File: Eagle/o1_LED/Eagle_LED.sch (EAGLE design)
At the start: 10 parts, among them Q1 S9013

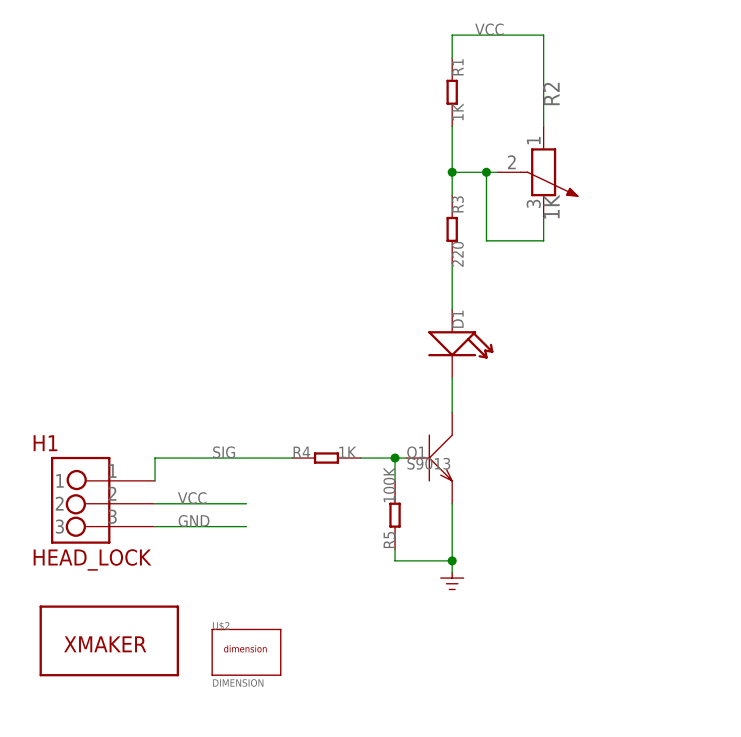
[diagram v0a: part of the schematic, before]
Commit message: miniuno
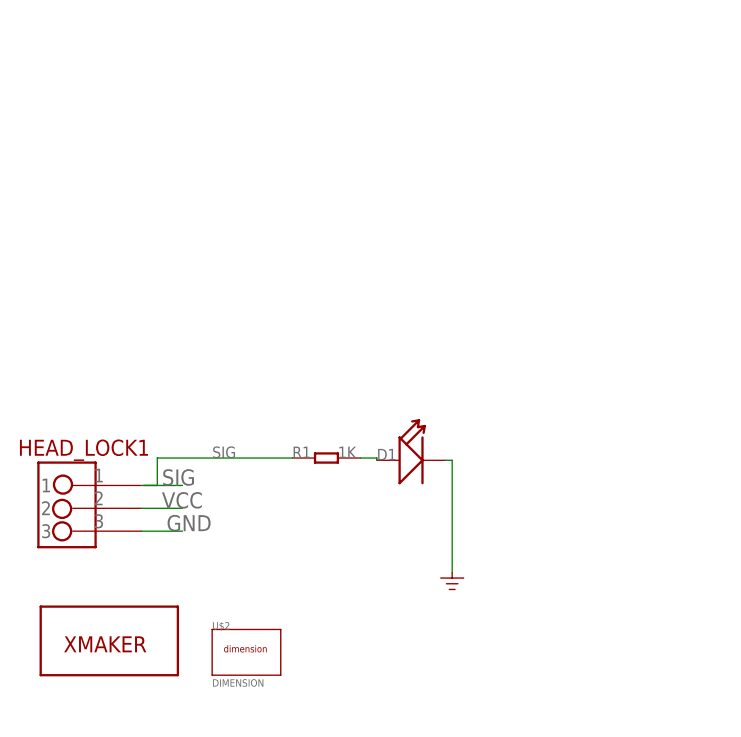
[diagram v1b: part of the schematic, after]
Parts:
- removed H1: HEAD_LOCK, HEAD_LOCK:HEAD_LOCK
- removed Q1: S9013, Discrete:TRANSISTOR-NPN-SOT23
- removed R2: 1K, Discrete:R-POTENTIOMETER'EVN-D8A-A03-B**'
- removed R3: 220, Discrete:005-R0603
- removed R4: 1K, Discrete:005-R0603
- removed R5: 100K, Discrete:005-R0603
- added HEAD_LOCK1: HEAD_LOCK, Xmaker_yuhuilbr:HEAD_LOCK
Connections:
- removed net N$2: D1.-, Q1.C
- removed net N$3: D1.+, R3.2
- removed net N$4: Q1.B, R4.2, R5.2
- net GND: now also D1.-, HEAD_LOCK1.3; no longer H1.3, Q1.E, R5.1
- net N$1: now also D1.+; no longer R2.2, R2.3, R3.1
- net SIG: now also HEAD_LOCK1.1, R1.1; no longer H1.1, R4.1
- net VCC: now also HEAD_LOCK1.2; no longer H1.2, R1.1, R2.1
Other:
- moved on the sheet: D1, R1
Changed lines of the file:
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@@
 <setting verticaltext="up"/>
 </settings>
-<grid distance="0.1" unitdist="inch" unit="inch" style="lines" multiple="1" display="no" altdistance="0.01" altunitdist="inch" altunit="inch"/>
+<grid distance="10" unitdist="mil" unit="mil" style="lines" multiple="1" display="no" altdistance="0.01" altunitdist="inch" altunit="inch"/>
 <layers>
 <layer number="1" name="Top" color="4" fill="1" visible="no" active="no"/>
@@
 <parts>
 <part name="U$1" library="moudle" deviceset="SEEEDSTUDIO_SCH_FRAME" device=""/>
+<part name="D1" library="Discrete" deviceset="LED*" device="-6MM"/>
+<part name="U$3" library="Power or GND " deviceset="GND_POWER" device=""/>
 <part name="R1" library="Discrete" deviceset="005-R*" device="0603" value="1K"/>
-<part name="D1" library="Discrete" deviceset="LED*" device="-6MM"/>
-<part name="R2" library="Discrete" deviceset="R-POTENTIOMETER*" device="'EVN-D8A-A03-B**'" value="1K"/>
-<part name="R3" library="Discrete" deviceset="005-R*" device="0603" value="220"/>
-<part name="Q1" library="Discrete" deviceset="TRANSISTOR-NPN*" device="-SOT23" value="S9013"/>
-<part name="U$3" library="Power or GND " deviceset="GND_POWER" device=""/>
-<part name="R4" library="Discrete" deviceset="005-R*" device="0603" value="1K"/>
-<part name="R5" library="Discrete" deviceset="005-R*" device="0603" value="100K"/>
-<part name="H1" library="HEAD_LOCK" deviceset="HEAD_LOCK" device=""/>
 <part name="U$4" library="switch-tact" deviceset="XMAKERLOGO" device=""/>
 <part name="U$2" library="Xmaker_yuhui" deviceset="DIMENSION" device=""/>
+<part name="HEAD_LOCK1" library="Xmaker_yuhuilbr" deviceset="HEAD_LOCK" device=""/>
 </parts>
 <sheets>
@@
 <instances>
 <instance part="U$1" gate="G$1" x="0" y="0"/>
-<instance part="R1" gate="R" x="129.54" y="105.41" rot="R270"/>
-<instance part="D1" gate="LED" x="129.54" y="77.47" rot="R270"/>
-<instance part="R2" gate="RP" x="139.7" y="96.52" rot="R270"/>
-<instance part="R3" gate="R" x="129.54" y="90.17" rot="R270"/>
-<instance part="Q1" gate="Q" x="127" y="64.77"/>
+<instance part="D1" gate="LED" x="124.968" y="64.516"/>
 <instance part="U$3" gate="G$1" x="129.54" y="52.07"/>
-<instance part="R4" gate="R" x="115.57" y="64.77"/>
-<instance part="R5" gate="R" x="123.19" y="58.42" rot="R90"/>
-<instance part="H1" gate="G$1" x="83.82" y="52.07"/>
+<instance part="R1" gate="R" x="115.57" y="64.77"/>
 <instance part="U$4" gate="G$1" x="91.44" y="43.18"/>
 <instance part="U$2" gate="G$1" x="106.68" y="43.18"/>
+<instance part="HEAD_LOCK1" gate="G$1" x="87.376" y="59.182"/>
 </instances>
 <busses>
 </busses>
 <nets>
+<net name="GND" class="0">
+<segment>
+<pinref part="D1" gate="LED" pin="-"/>
+<pinref part="U$3" gate="G$1" pin="GND"/>
+<wire x1="128.778" y1="64.516" x2="129.54" y2="64.516" width="0.1524" layer="91"/>
+<wire x1="129.54" y1="64.516" x2="129.54" y2="52.07" width="0.1524" layer="91"/>
+</segment>
+<segment>
+<wire x1="94.996" y1="56.642" x2="99.568" y2="56.642" width="0.1524" layer="91"/>
+<label x="97.79" y="56.642" size="1.778" layer="95"/>
+<pinref part="HEAD_LOCK1" gate="G$1" pin="3"/>
+</segment>
+</net>
+<net name="SIG" class="0">
+<segment>
+<label x="102.87" y="64.77" size="1.27" layer="95" ratio="10"/>
+<pinref part="R1" gate="R" pin="1"/>
+<wire x1="96.774" y1="64.77" x2="111.76" y2="64.77" width="0.1524" layer="91"/>
+<wire x1="95.25" y1="61.722" x2="96.774" y2="61.722" width="0.1524" layer="91"/>
+<wire x1="96.774" y1="61.722" x2="96.774" y2="64.77" width="0.1524" layer="91"/>
+</segment>
+<segment>
+<pinref part="HEAD_LOCK1" gate="G$1" pin="1"/>
+<wire x1="94.996" y1="61.722" x2="99.568" y2="61.722" width="0.1524" layer="91"/>
+<label x="97.282" y="61.722" size="1.778" layer="95"/>
+</segment>
+</net>
 <net name="N$1" class="0">
 <segment>
-<wire x1="129.54" y1="101.6" x2="129.54" y2="96.52" width="0.1524" layer="91"/>
 <pinref part="R1" gate="R" pin="2"/>
-<pinref part="R2" gate="RP" pin="3"/>
-<wire x1="134.62" y1="96.52" x2="133.35" y2="96.52" width="0.1524" layer="91"/>
-<pinref part="R3" gate="R" pin="1"/>
-<wire x1="133.35" y1="96.52" x2="129.54" y2="96.52" width="0.1524" layer="91"/>
-<wire x1="129.54" y1="93.98" x2="129.54" y2="96.52" width="0.1524" layer="91"/>
-<junction x="129.54" y="96.52"/>
-<pinref part="R2" gate="RP" pin="2"/>
-<wire x1="139.7" y1="91.44" x2="139.7" y2="88.9" width="0.1524" layer="91"/>
-<wire x1="139.7" y1="88.9" x2="133.35" y2="88.9" width="0.1524" layer="91"/>
-<wire x1="133.35" y1="88.9" x2="133.35" y2="96.52" width="0.1524" layer="91"/>
-<junction x="133.35" y="96.52"/>
-</segment>
-</net>
-<net name="GND" class="0">
-<segment>
-<wire x1="96.52" y1="57.15" x2="106.68" y2="57.15" width="0.1524" layer="91"/>
-<label x="99.06" y="57.15" size="1.27" layer="95"/>
-<pinref part="H1" gate="G$1" pin="3"/>
-</segment>
-<segment>
-<pinref part="U$3" gate="G$1" pin="GND"/>
-<pinref part="Q1" gate="Q" pin="E"/>
-<wire x1="129.54" y1="52.07" x2="129.54" y2="53.34" width="0.1524" layer="91"/>
-<pinref part="R5" gate="R" pin="1"/>
-<wire x1="129.54" y1="53.34" x2="129.54" y2="59.69" width="0.1524" layer="91"/>
-<wire x1="123.19" y1="54.61" x2="123.19" y2="53.34" width="0.1524" layer="91"/>
-<wire x1="129.54" y1="53.34" x2="123.19" y2="53.34" width="0.1524" layer="91"/>
-<junction x="129.54" y="53.34"/>
+<pinref part="D1" gate="LED" pin="+"/>
+<wire x1="119.38" y1="64.77" x2="121.158" y2="64.77" width="0.1524" layer="91"/>
+<wire x1="121.158" y1="64.77" x2="121.158" y2="64.516" width="0.1524" layer="91"/>
 </segment>
 </net>
 <net name="VCC" class="0">
 <segment>
-<wire x1="96.52" y1="59.69" x2="106.68" y2="59.69" width="0.1524" layer="91"/>
-<label x="99.06" y="59.69" size="1.27" layer="95"/>
-<pinref part="H1" gate="G$1" pin="2"/>
-</segment>
-<segment>
-<pinref part="R2" gate="RP" pin="1"/>
-<wire x1="139.7" y1="101.6" x2="139.7" y2="111.76" width="0.1524" layer="91"/>
-<pinref part="R1" gate="R" pin="1"/>
-<wire x1="139.7" y1="111.76" x2="129.54" y2="111.76" width="0.1524" layer="91"/>
-<wire x1="129.54" y1="111.76" x2="129.54" y2="109.22" width="0.1524" layer="91"/>
-<label x="132.08" y="111.76" size="1.27" layer="95" ratio="10"/>
-</segment>
-</net>
-<net name="N$3" class="0">
-<segment>
-<pinref part="R3" gate="R" pin="2"/>
-<wire x1="129.54" y1="86.36" x2="129.54" y2="81.28" width="0.1524" layer="91"/>
-<pinref part="D1" gate="LED" pin="+"/>
-</segment>
-</net>
-<net name="SIG" class="0">
-<segment>
-<wire x1="96.52" y1="64.77" x2="111.76" y2="64.77" width="0.1524" layer="91"/>
-<label x="102.87" y="64.77" size="1.27" layer="95" ratio="10"/>
-<pinref part="R4" gate="R" pin="1"/>
-<wire x1="96.52" y1="62.23" x2="96.52" y2="64.77" width="0.1524" layer="91"/>
-<pinref part="H1" gate="G$1" pin="1"/>
-</segment>
-</net>
-<net name="N$2" class="0">
-<segment>
-<pinref part="Q1" gate="Q" pin="C"/>
-<pinref part="D1" gate="LED" pin="-"/>
-<wire x1="129.54" y1="69.85" x2="129.54" y2="73.66" width="0.1524" layer="91"/>
-</segment>
-</net>
-<net name="N$4" class="0">
-<segment>
-<pinref part="Q1" gate="Q" pin="B"/>
-<pinref part="R4" gate="R" pin="2"/>
-<wire x1="124.46" y1="64.77" x2="123.19" y2="64.77" width="0.1524" layer="91"/>
-<pinref part="R5" gate="R" pin="2"/>
-<wire x1="123.19" y1="64.77" x2="119.38" y2="64.77" width="0.1524" layer="91"/>
-<wire x1="123.19" y1="62.23" x2="123.19" y2="64.77" width="0.1524" layer="91"/>
-<junction x="123.19" y="64.77"/>
-</segment>
-</net>
+<pinref part="HEAD_LOCK1" gate="G$1" pin="2"/>
+<wire x1="94.996" y1="59.182" x2="99.568" y2="59.182" width="0.1524" layer="91"/>
+<label x="97.282" y="59.182" size="1.778" layer="95"/>
+</segment>
+</net>
